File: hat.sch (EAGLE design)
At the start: 13 parts, among them U1 HEX_CONVERTER

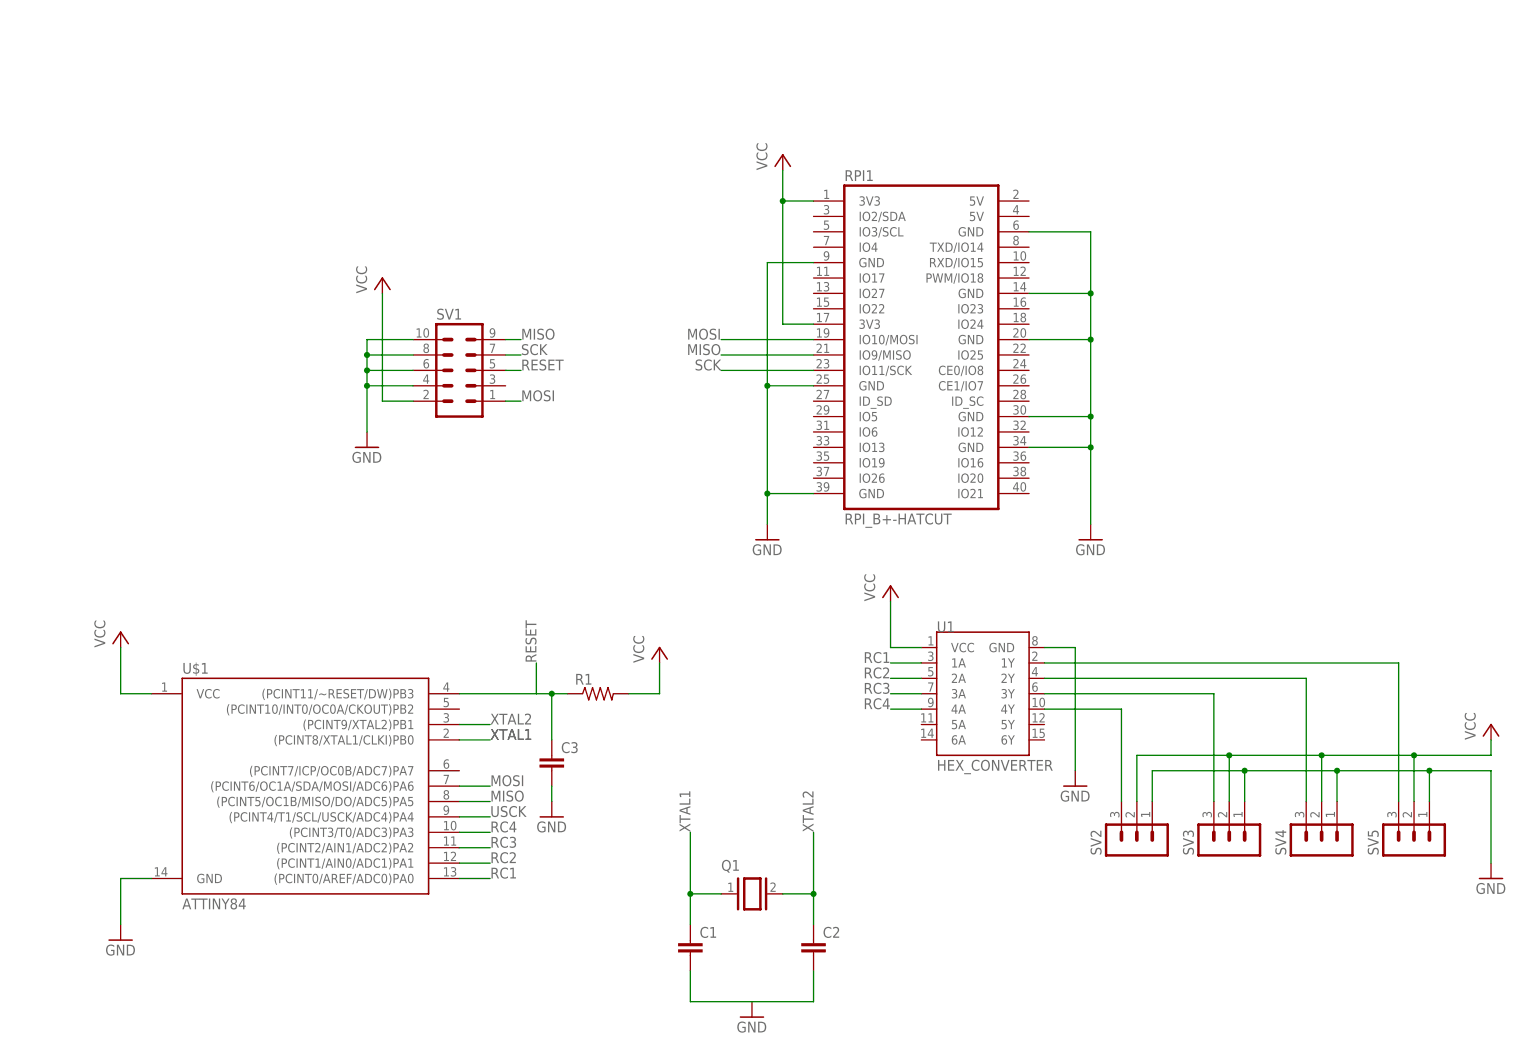
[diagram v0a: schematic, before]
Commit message: Work in progess
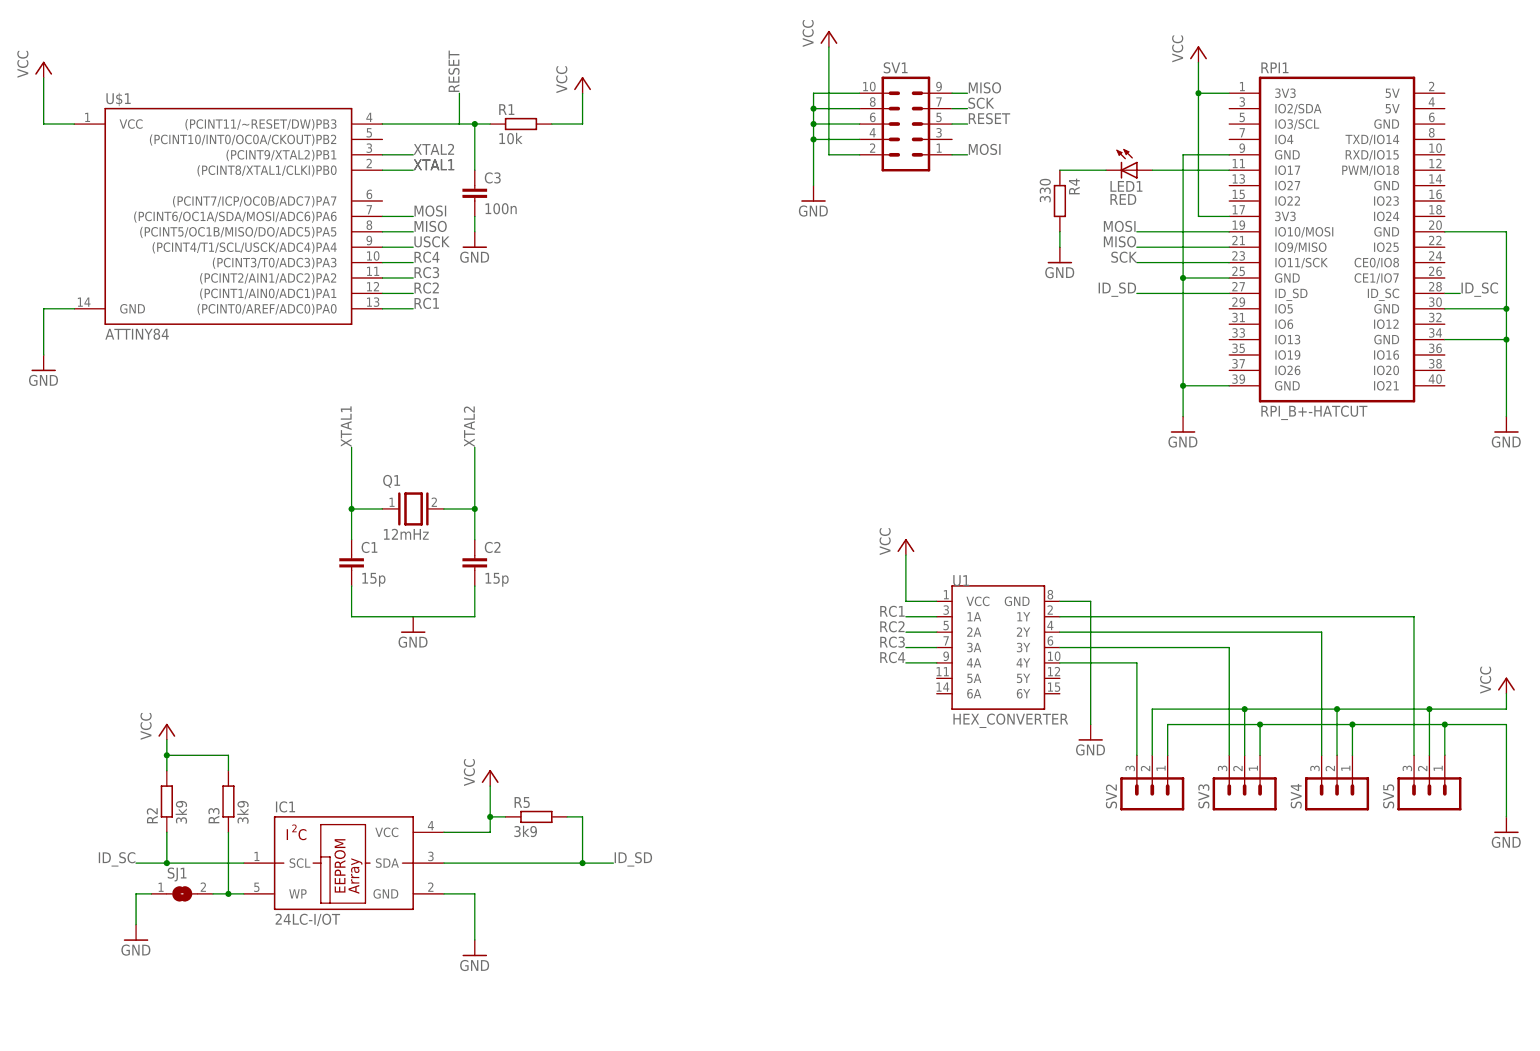
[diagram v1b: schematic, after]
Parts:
- added IC1: 24LC-I/OT, we-chip:24LC-I/OT
- added LED1: RED, led:LEDCHIPLED_0805
- added R2, R3, R5: 3k9, resistor:R-EU_R0805
- added R4: 330, rcl:R-EU_R0805
- added SJ1: (no value), jumper:SJ
- C1, C2: value (none) -> 15p
- C3: value (none) -> 100n
- Q1: value (none) -> 12mHz
- R1: value (none) -> 10k; device SparkFun-Resistors:RESISTOR1206 -> resistor:R-EU_R0805
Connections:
- new net ID_SC: IC1.SCL, R2.1, RPI1.ID_SC
- new net ID_SD: IC1.SDA, R5.2, RPI1.ID_SD
- new net N$5: IC1.WP, R3.1, SJ1.2
- new net N$7: LED1.A, RPI1.IO17
- new net N$8: LED1.C, R4.1
- net GND: now also IC1.GND, R4.2, SJ1.1; no longer RPI1.GND@1, RPI1.GND@3
- net VCC: now also IC1.VCC, R2.2, R3.2, R5.1
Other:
- moved on the sheet: C1, C2, C3, Q1, RPI1, SV1, SV2, SV3, SV4, SV5, U$1, U1
